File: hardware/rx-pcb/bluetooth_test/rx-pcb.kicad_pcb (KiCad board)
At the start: 4 copper layers, 23.1 x 37.6 mm, 43 parts, among them J1 Conn_01x05_Pin, J2 Conn_01x04_Pin, J3 Conn_Coaxial_Small, J4 Conn_01x04_Pin, J5 Conn_01x02_Pin, J6 Conn_01x02_Pin, SW1 SW_SPST, U1 STM32WB05KZV6TR, U2 STS4L-AD1B-R3, U3 LMT70AYFQR, X1 Q22FA12800025, X2 ABS07-32.768KHZ-1-T

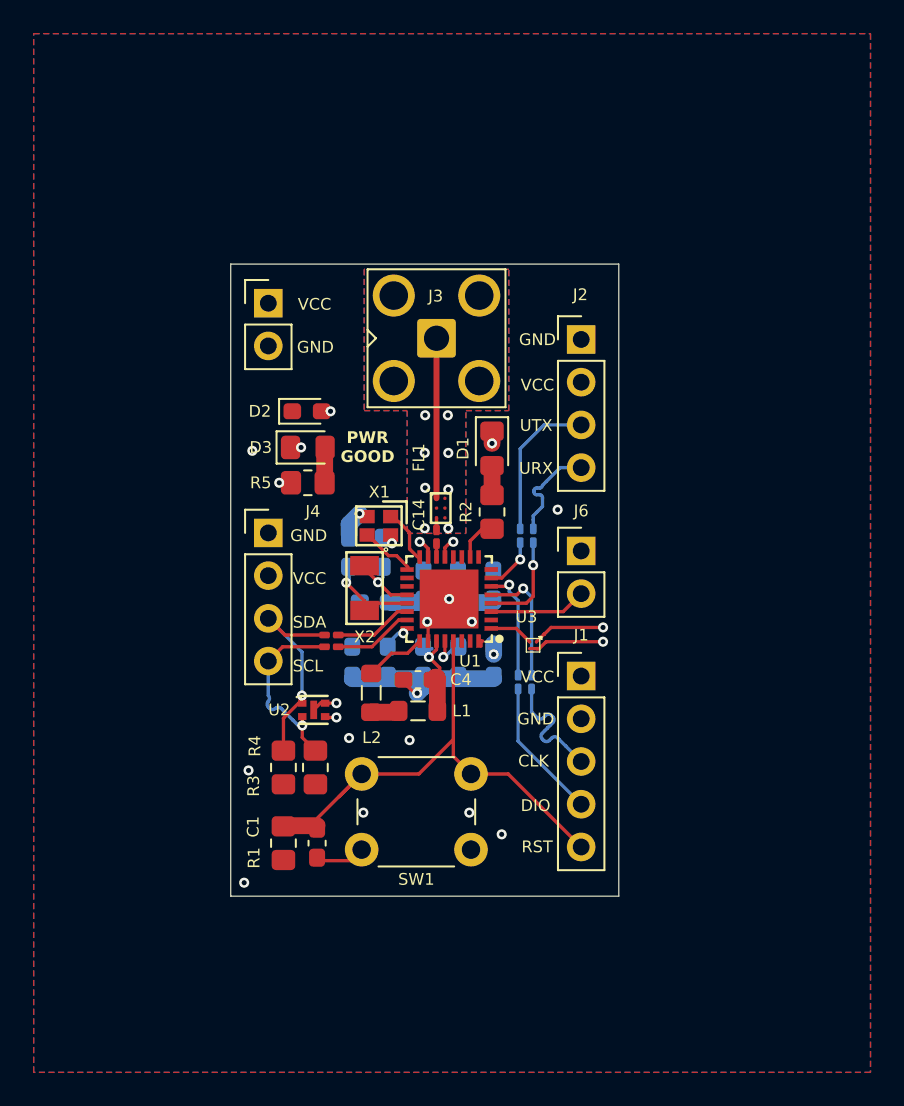
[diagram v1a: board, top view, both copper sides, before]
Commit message: updates for dr weeks
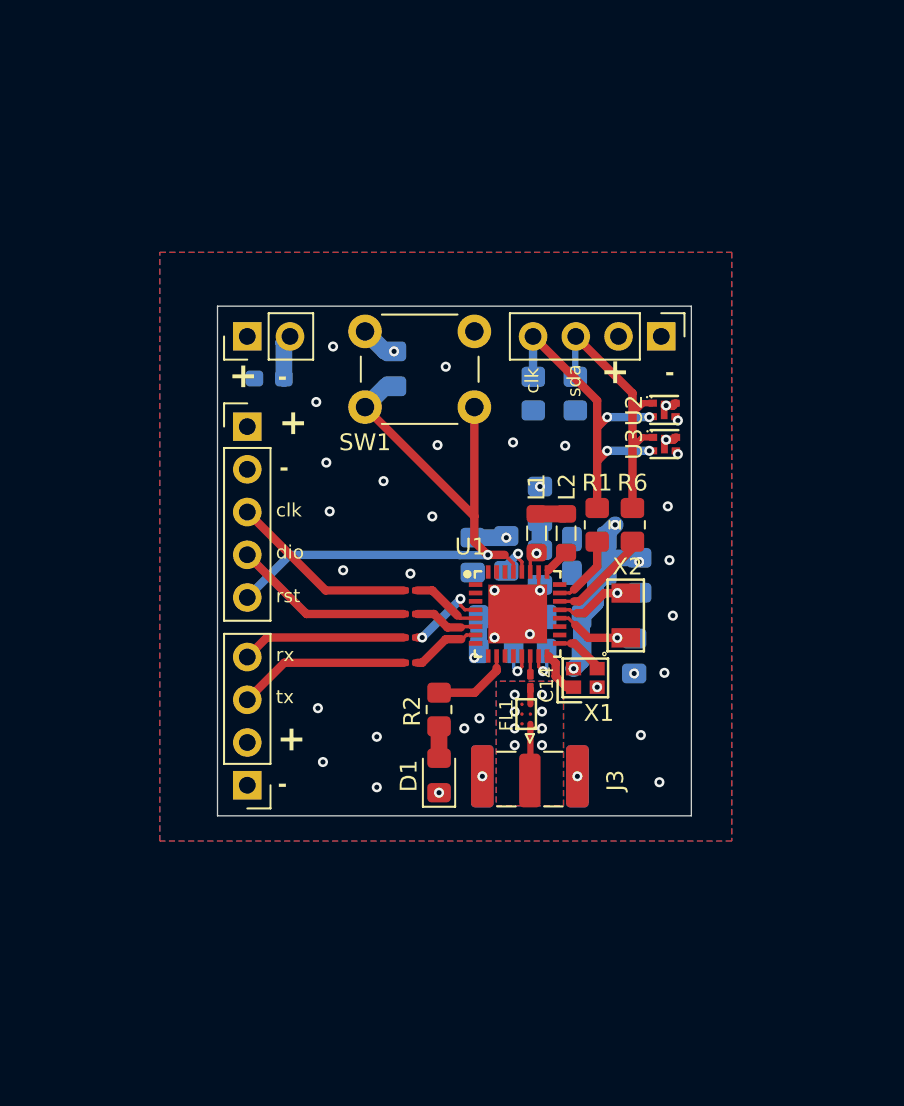
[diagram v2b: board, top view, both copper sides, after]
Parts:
- removed D3: LED, rx-parts:LED_0805_2012Metric_Pad1.15x1.40mm_HandSolder
- removed J6: Conn_01x02_Pin, Connector_PinHeader_2.54mm:PinHeader_1x02_P2.54mm_Vertical
- removed the R1 at (148.2, 104.5)
- removed the R1 at (145.3, 116.1)
- removed R5: 10k, rx-parts:R_0805_2012Metric_Pad1.20x1.40mm_HandSolder
- added R1: 0, Resistor_SMD:R_0805_2012Metric_Pad1.20x1.40mm_HandSolder, F.Cu at (164.0, 97.2)
- C1, C4: footprint Capacitor_SMD:C_0603_1608Metric_Pad1.08x0.95mm_HandSolder -> Capacitor_SMD:C_0805_2012Metric_Pad1.18x1.45mm_HandSolder; moved to B.Cu
- C10, C11, C12, C13, C2, C3, C5, C6, C7, C8, C9: footprint Capacitor_SMD:C_0603_1608Metric_Pad1.08x0.95mm_HandSolder -> Capacitor_SMD:C_0805_2012Metric_Pad1.18x1.45mm_HandSolder
- D2, R3, R4: moved to B.Cu
- J3: footprint rx-parts:SMA_Amphenol_901-143_Horizontal -> Connector_Coaxial:SMA_Samtec_SMA-J-P-H-ST-EM1_EdgeMount
- R10, R7, R8, R9: moved to F.Cu
- R6: footprint Resistor_SMD:R_0201_0603Metric_Pad0.64x0.40mm_HandSolder -> Resistor_SMD:R_0805_2012Metric_Pad1.20x1.40mm_HandSolder
- U3: value LMT70AYFQR -> STS4L-AD1B-R3; footprint rx-parts:DSBGA-4_L0.8-W0.8-R2-C2-P0.40-BL -> rx-parts:DFN-4_L1.5-W1.5-P0.80-TL-EP
- moved J2 33.1 mm to (143.2, 112.7), turned to 180 degrees
- moved SW1 31.4 mm to (150.2, 85.7), turned to 0 degrees
- moved C1 28.6 mm to (151.9, 87.9), turned to 90 degrees
- moved R4 28.2 mm to (162.7, 89.4)
- moved U2 27.4 mm to (168.0, 90.4)
- moved J3 26.9 mm to (160.0, 112.4), turned to -90 degrees
- moved J4 26.1 mm to (167.8, 86.0), turned to -90 degrees
- moved R3 25.7 mm to (160.2, 89.4)
- moved J1 24.8 mm to (143.2, 91.4)
- moved D1 19.7 mm to (154.6, 112.1), turned to 90 degrees
- moved R6 19.1 mm to (166.1, 97.2), turned to -90 degrees
- moved C3 17.3 mm to (166.5, 100.2)
- moved C2 16.2 mm to (166.2, 105.0), turned to -90 degrees
- moved C11 15.9 mm to (163.5, 98.0), turned to 0 degrees
- moved X2 15.6 mm to (165.7, 102.6), turned to 90 degrees
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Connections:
- U1 pad 3: /ADC_jump -> unconnected-(U1-PB1-Pad3)
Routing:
- net /i2c_scl: track 11.4 -> 21.0 mm, vias 1 -> 4
- net GND: track 30.5 -> 22.8 mm, vias 22 -> 38
- net /rst: track 31.3 -> 38.1 mm, vias 0 -> 1
- net /ANT: track 9.52 -> 3.38 mm
- net VCC: track 10.4 -> 4.60 mm, vias 13 -> 16
- net /ADC_jump: track 5.79 -> 0.00 mm
- net /i2c_sda: track 13.0 -> 17.0 mm, vias 1 -> 0
- net /swclk: track 7.62 -> 11.2 mm
- net /uart_rx: track 6.27 -> 9.77 mm
- net Net-(U1-PA3): track 7.42 -> 4.15 mm, vias 1 -> 0
- net Net-(U1-PA2): track 6.72 -> 3.82 mm, vias 1 -> 0
- net /TMP_A: track 2.62 -> 0.00 mm
- net /swdio: track 8.41 -> 10.8 mm
- net /vlxsd: track 3.68 -> 1.47 mm
- net Net-(D3-A): track 2.11 -> 0.00 mm
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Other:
- board size 23.1 x 37.6 mm -> 28.2 x 30.3 mm
- board text added: "+"
- board text added: "-"
- board text added: "clk"
- board text added: "dio"
- board text added: "rst"
- board text added: "rx"
- board text added: "sda"
- board text added: "tx"
- board text removed: "CLK"
- board text removed: "DIO"
- board text removed: "GND"
- board text removed: "PWR GOOD"
- board text removed: "RST"
- board text removed: "SCL"
- board text removed: "SDA"
- board text removed: "URX"
- board text removed: "UTX"
- board text removed: "VCC"
- board text removed: "trace impedance based upon: JLC04161H-7628(Standard/Finished thickness1.59mm±10%)"
